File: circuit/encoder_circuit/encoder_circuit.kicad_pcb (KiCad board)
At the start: 2 copper layers, 27 x 23 mm, 9 parts, among them J1 Conn_01x04

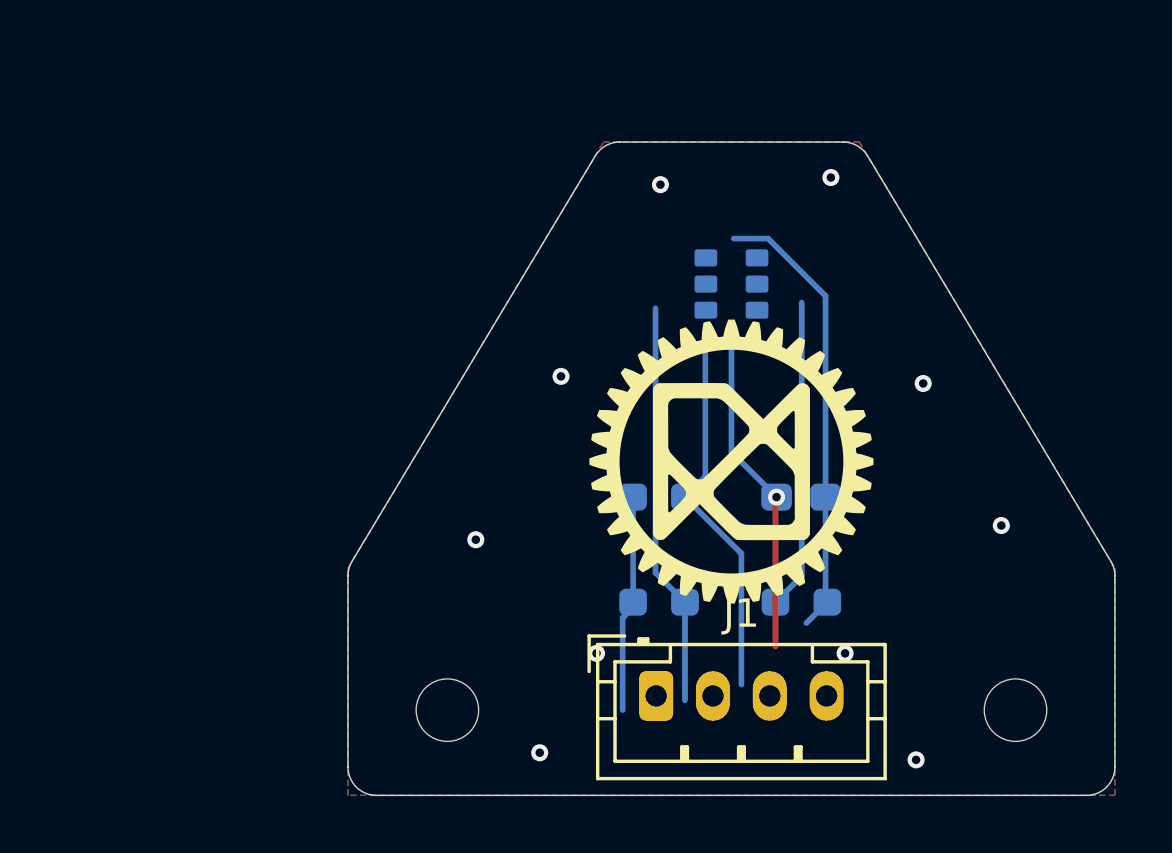
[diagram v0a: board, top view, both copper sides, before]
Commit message: エンコーダ基板修正
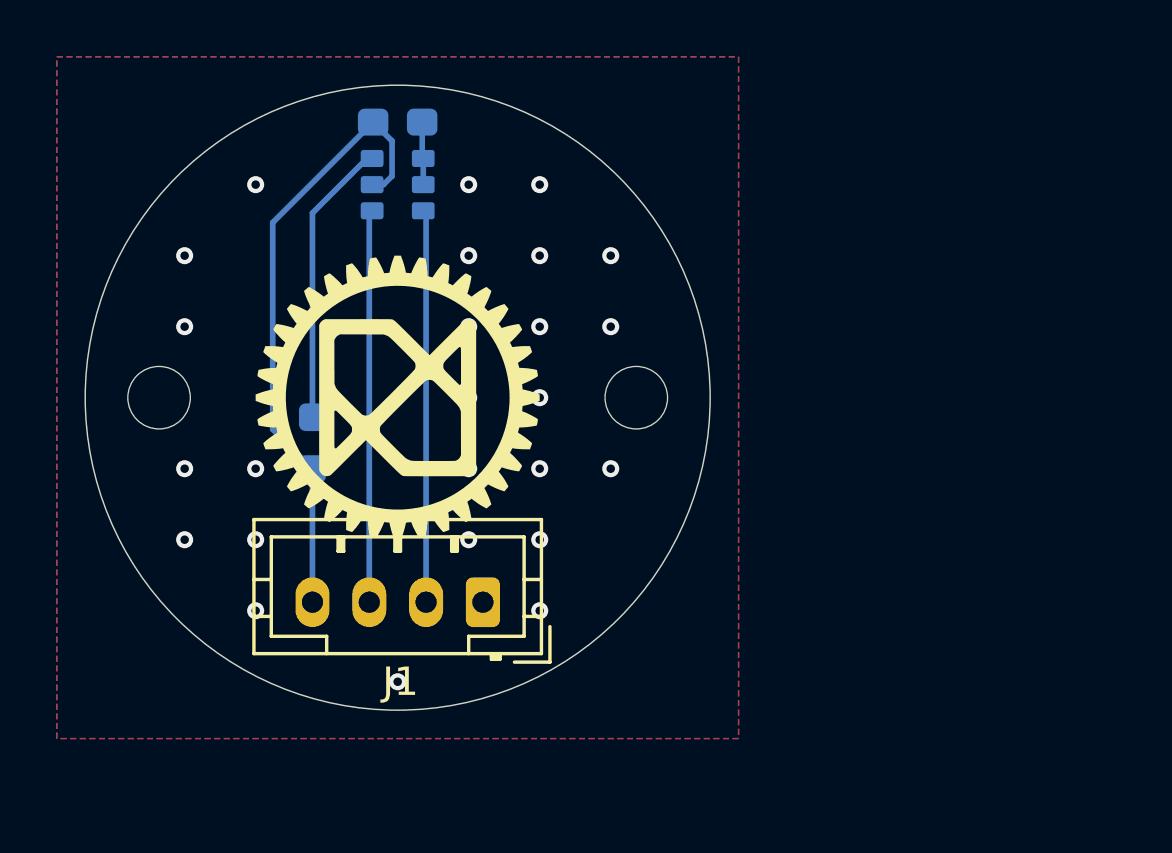
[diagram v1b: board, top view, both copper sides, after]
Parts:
- removed R2, R3: 1k, Resistor_SMD:R_0603_1608Metric_Pad0.98x0.95mm_HandSolder
- removed the REF** at (131.8, 101.0)
- removed the REF** at (151.8, 101.0)
- added REF**: MountingHole_2.2mm_M2, MountingHole:MountingHole_2.2mm_M2, F.Cu at (121.6, 90.0)
- added REF**: MountingHole_2.2mm_M2, MountingHole:MountingHole_2.2mm_M2, F.Cu at (138.4, 90.0)
- moved C1 19.4 mm to (130.0, 80.3), turned to 0 degrees
- moved R1 18.1 mm to (127.0, 91.6), turned to 90 degrees
- moved U1 12.3 mm to (130.0, 82.5)
- moved G*** 12.0 mm to (130.0, 90.0)
- moved J1 6.94 mm to (133.0, 97.2), turned to 180 degrees
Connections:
- J1 pad 1: +3.3V -> GND
- J1 pad 4: GND -> +3.3V
- U1 pad 3: Net-(J1-Pin_3) -> Net-(J1-Pin_2)
- U1 pad 4: Net-(J1-Pin_2) -> Net-(J1-Pin_3)
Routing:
- net GND: track 11.4 -> 2.22 mm, vias 11 -> 25
- net +3.3V: track 23.6 -> 22.1 mm
- net Net-(U1-Anode): track 10.9 -> 10.1 mm
- net Net-(J1-Pin_3): track 13.1 -> 13.8 mm
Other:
- board size 27 x 23 mm -> 22 x 22 mm
